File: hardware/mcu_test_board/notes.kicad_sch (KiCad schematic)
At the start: 0 parts

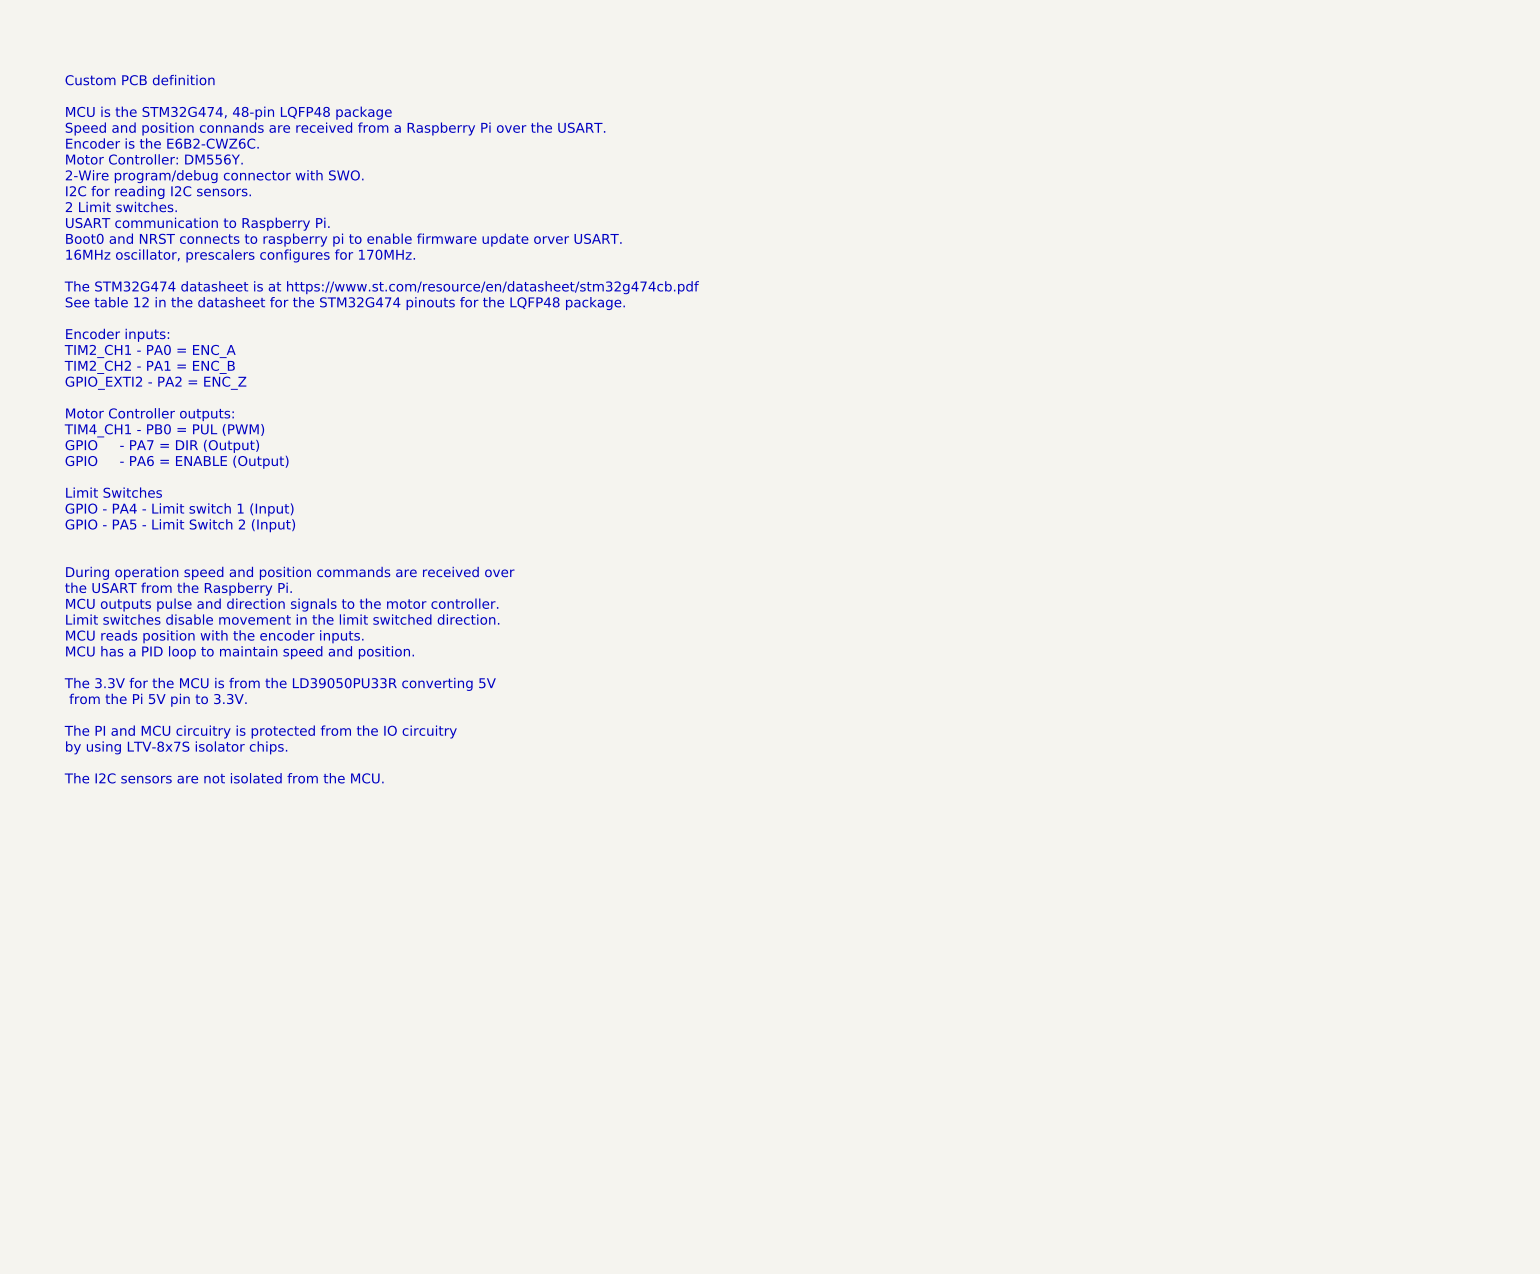
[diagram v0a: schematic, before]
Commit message: Latest mcu_test_board
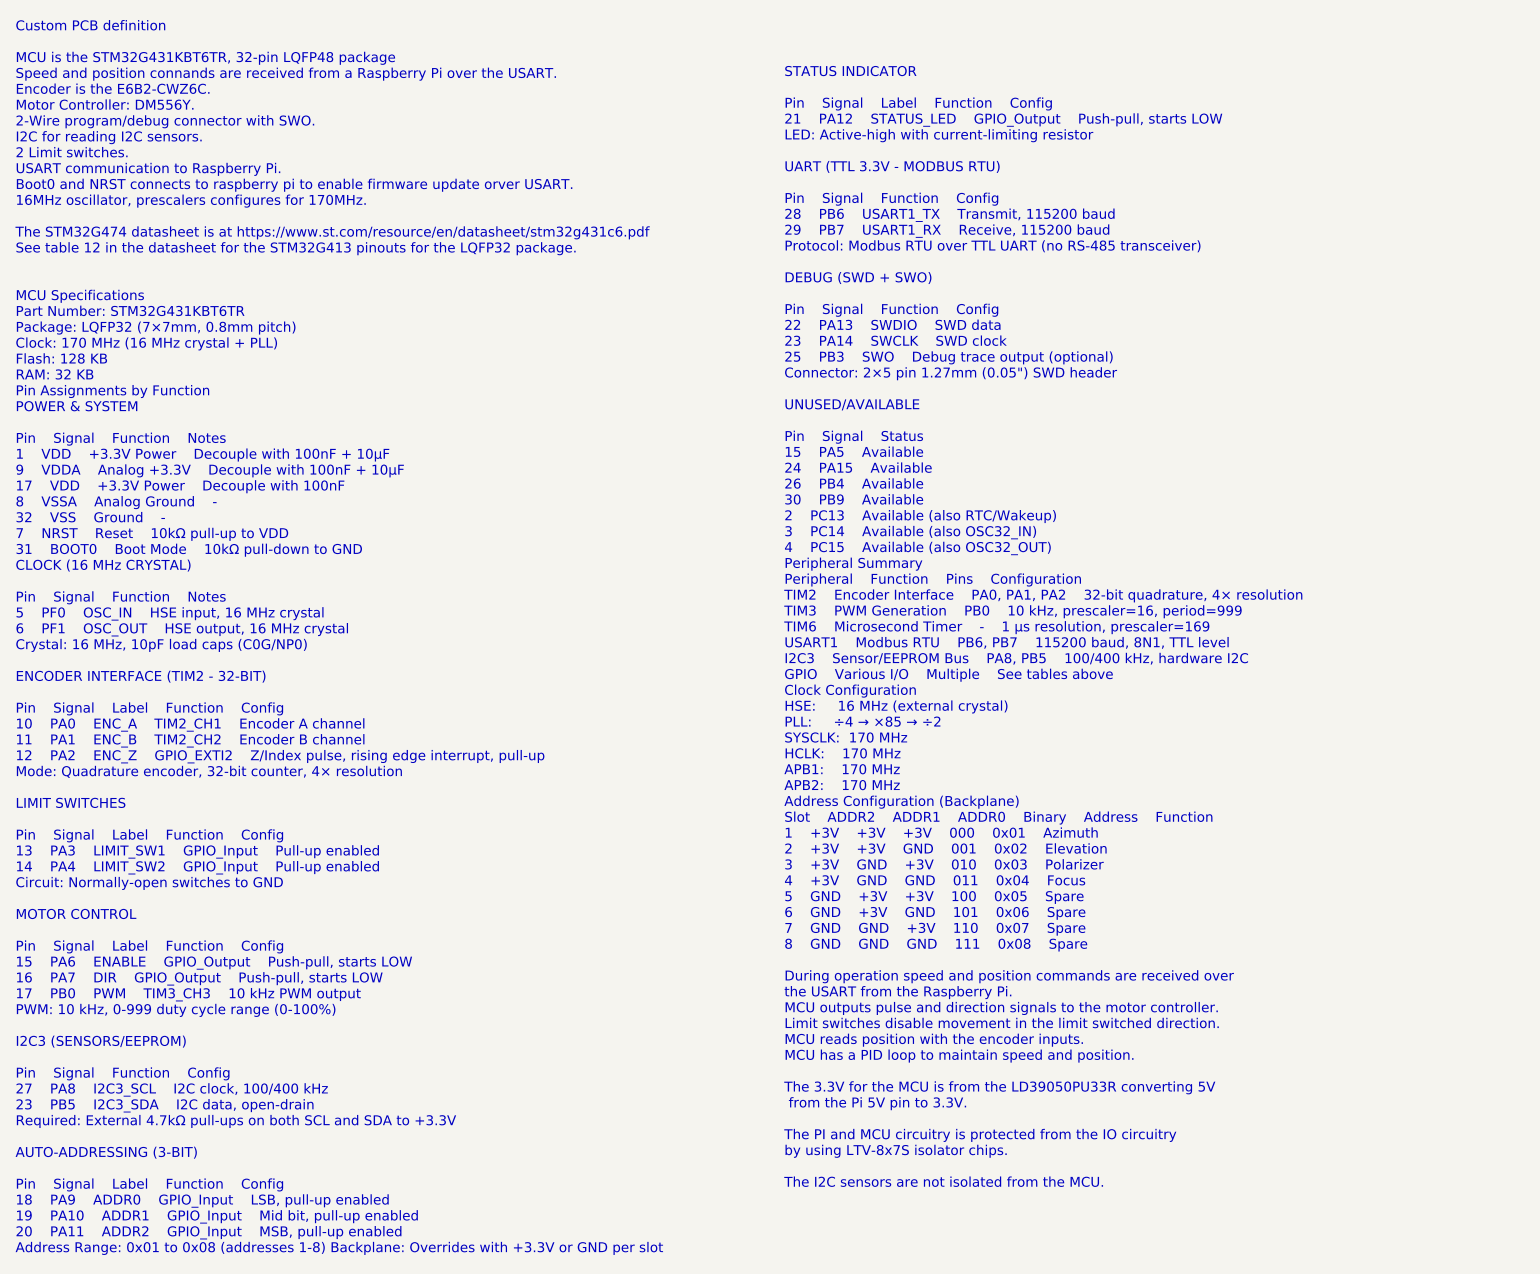
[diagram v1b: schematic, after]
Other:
- note added: "Custom PCB definition MCU is the STM32G431KBT6TR, 32-pin LQFP48 package Speed and position connands are received from a Raspberry Pi over the USART. Encoder is the E6B2-CWZ6C. Motor Controller: DM556Y. 2-Wire program/debug connector with SWO. I2C for reading I2C sensors. 2 Limit switches. USART communication to Raspberry Pi. Boot0 and NRST connects to raspberry pi to enable firmware update orver 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"
- note added: "STATUS INDICATOR Pin Signal Label Function Config 21 PA12 STATUS_LED GPIO_Output Push-pull, starts LOW LED: Active-high with current-limiting resistor UART (TTL 3.3V - MODBUS RTU) Pin Signal Function Config 28 PB6 USART1_TX Transmit, 115200 baud 29 PB7 USART1_RX Receive, 115200 baud Protocol: Modbus RTU over TTL UART (no RS-485 transceiver) DEBUG (SWD + SWO) Pin Signal Function Config 22 PA13 SWD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"
- note removed: "Custom PCB definition MCU is the STM32G474, 48-pin LQFP48 package Speed and position connands are received from a Raspberry Pi over the USART. Encoder is the E6B2-CWZ6C. Motor Controller: DM556Y. 2-Wire program/debug connector with SWO. I2C for reading I2C sensors. 2 Limit switches. USART communication to Raspberry Pi. Boot0 and NRST connects to raspberry pi to enable firmware update orver USART.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"
